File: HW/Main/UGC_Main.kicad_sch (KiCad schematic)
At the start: 128 parts, among them J1 Rumble, J13 503480-0640, J2 LT, J3 RT, J4 Conn_01x06_Pin, J5 UJ31-CH-G1-SMT-TR, Q1 MMBT3904, Q2 MMBT3904, Q3 BSS138DW, Q4 BSS138DW, Q5 Q_NMOS_GSD, Q6 Q_PMOS_GDS, Q7 Q_NMOS_GSD, SW1 1TS026A-1000-0550, SW1 SW_Push, SW10 SW_Push, SW11 SW_Push, SW12 SW_Push, SW13 SW_Push, SW14 TS09-63-25-R-260-SMT, SW2 SW_Push, SW3 SW_Push, SW4 SW_Push, SW5 SW_Push, SW6 GL18_SW, SW7 SW_Push, SW8 SW_Push, SW9 TS09-63-25-R-260-SMT, U1 ESP32-PICO-MINI-02, U10 ST_LSM6, U11 BQ25180, U12 CH340K, U13 PI3USB4000A, U2 GD25Q80EEIGR, U2 GH39F (Hall SOT23), U3 GH39F (Hall SOT23), U4 TPS630001RCR, U5 ST_LSM6, U6 MCP3002, U7 MCP3002, U8 RP2040, Y1 Crystal_GND3

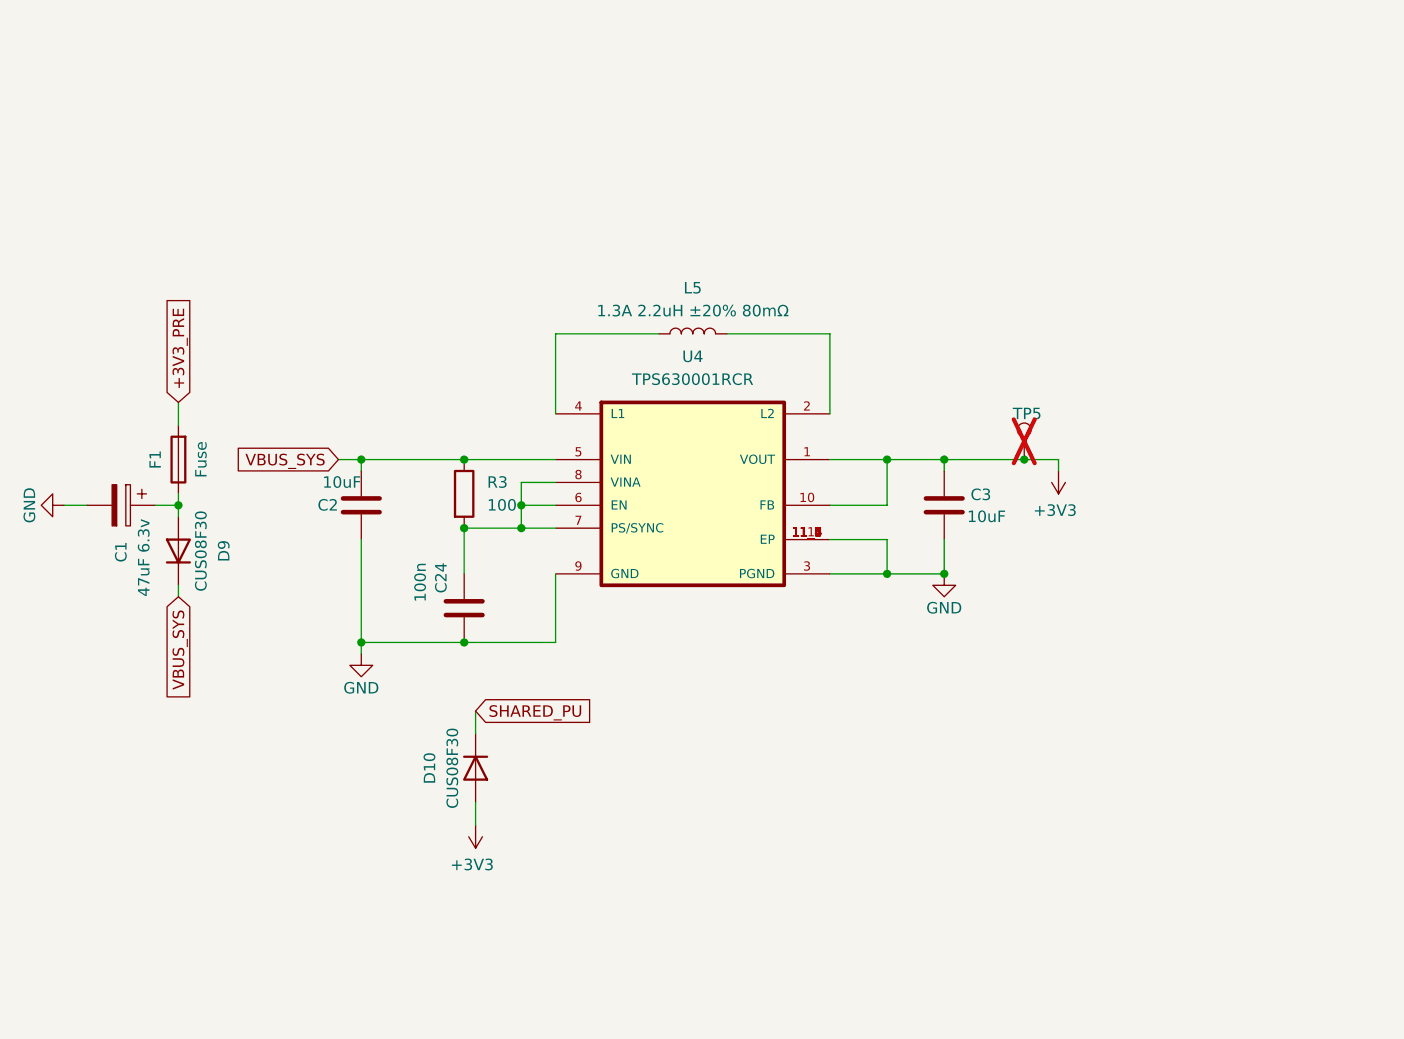
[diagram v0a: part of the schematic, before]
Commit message: Update board
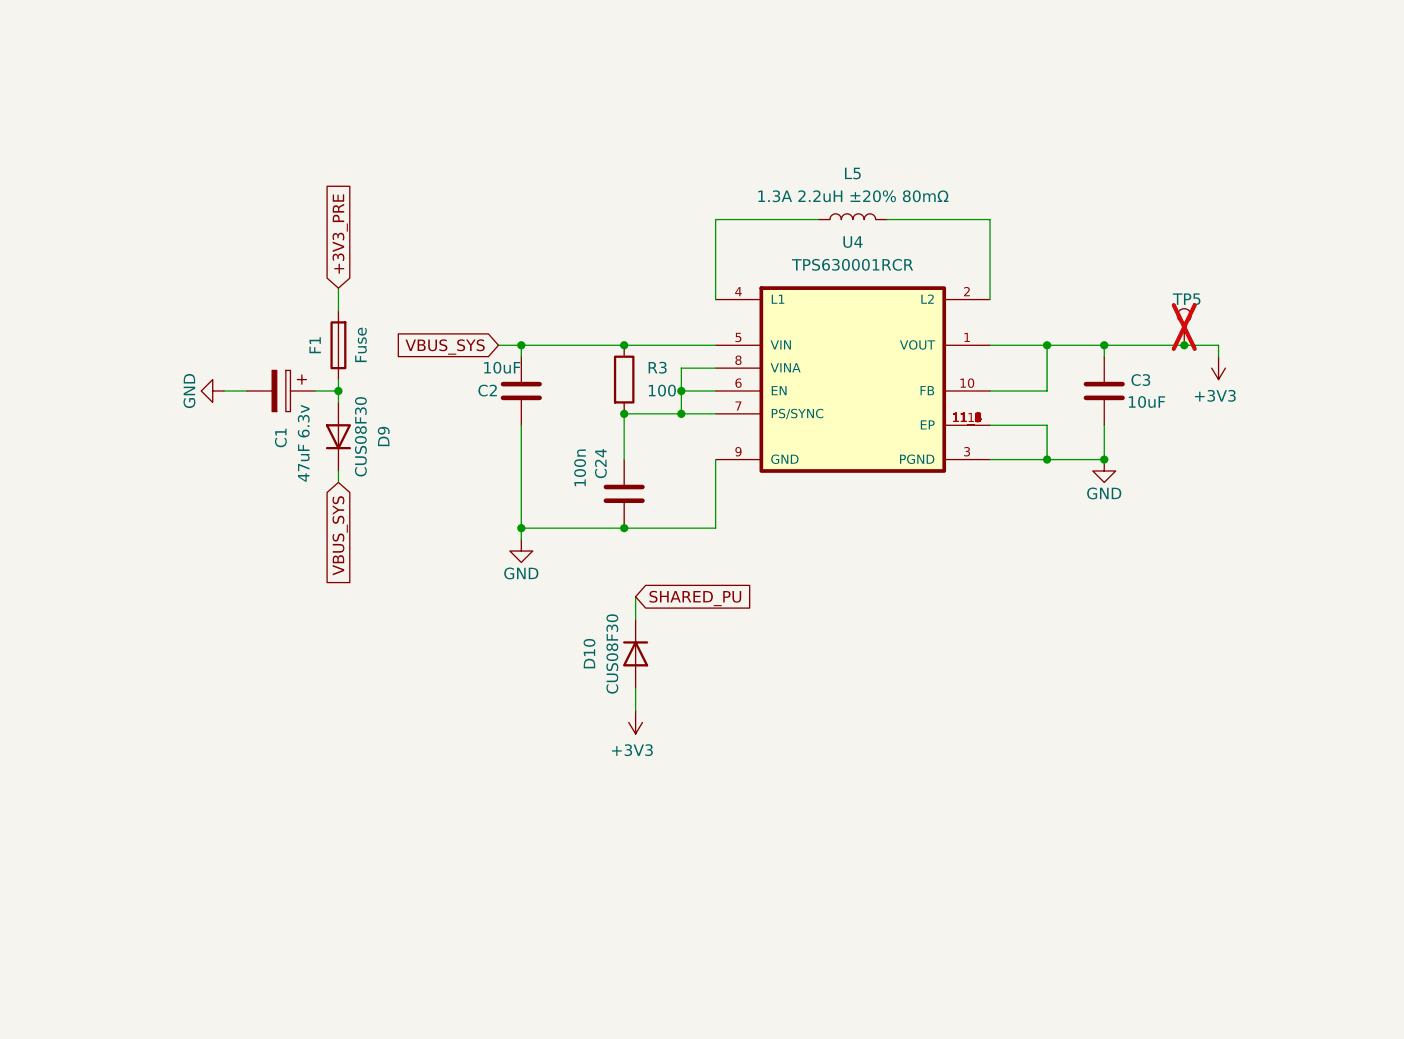
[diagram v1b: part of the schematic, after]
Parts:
- SW1, SW2, SW3, SW4: footprint hhl:progcc_bpad -> hhl:ring_pad
- SW10, SW11, SW12, SW13: footprint hhl:progcc_dpad -> hhl:ring_dpad
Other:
- moved on the sheet: C1, C2, C24, C3, D10, D9, F1, L5, R3, TP5, U4
